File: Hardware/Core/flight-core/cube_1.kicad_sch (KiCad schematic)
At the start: 18 parts, among them J10 Conn_02x06_Counter_Clockwise, J11 Conn_01x04_Socket, J501 Conn_02x02_Counter_Clockwise, J502 Conn_01x04_Socket, J503 Conn_01x03, J9 Cube Orange Plus Female Header, Q3 MMBF170, Q501 MMBF170, Q502 MMBF170

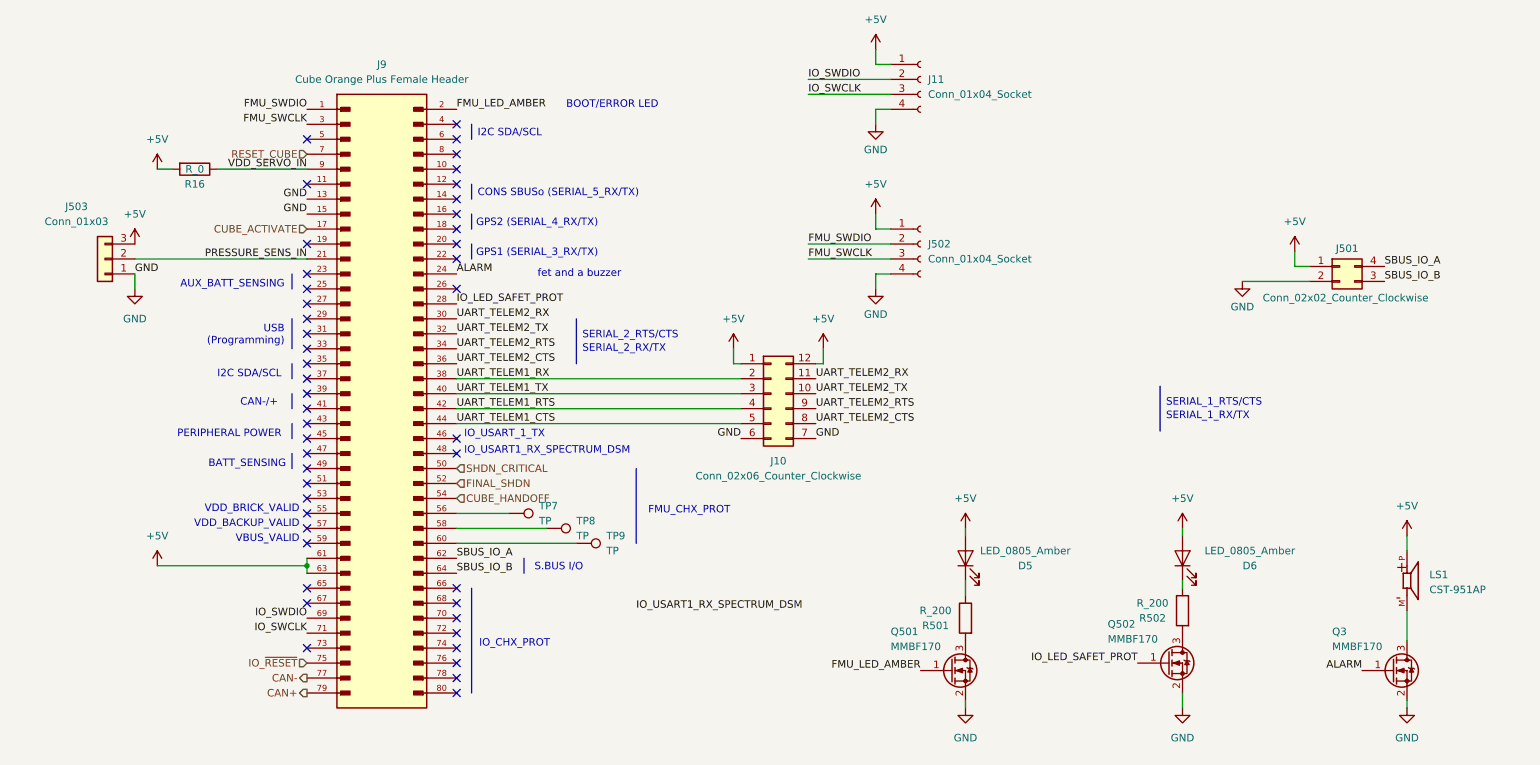
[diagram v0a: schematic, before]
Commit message: minor reformatting; no substantial changes
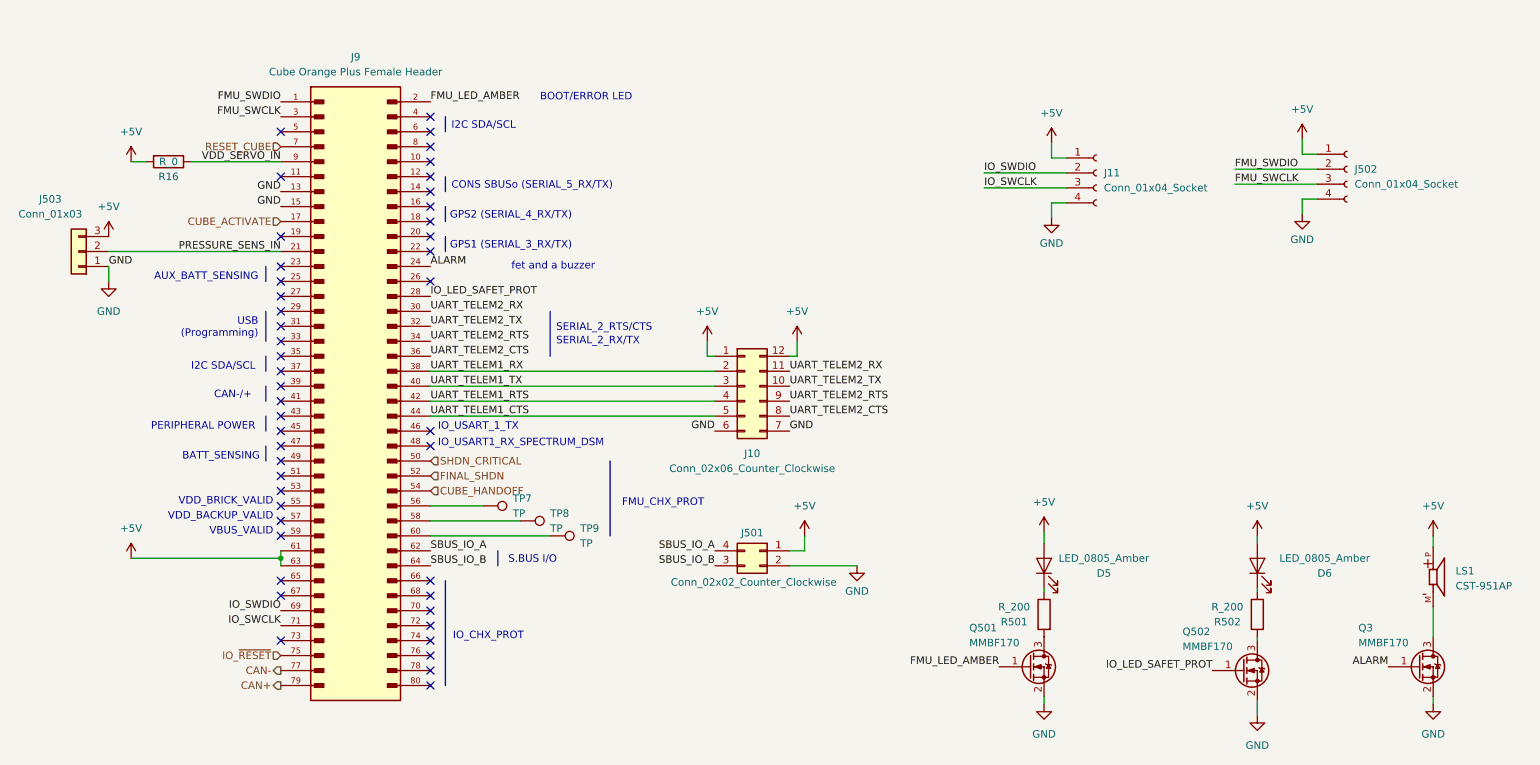
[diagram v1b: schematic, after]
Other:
- note removed: "SERIAL_1_RTS/CTS"
- note removed: "SERIAL_1_RX/TX"
- moved on the sheet: D5, D6, J10, J11, J501, J502, J503, J9, LS1, Q3, Q501, Q502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
